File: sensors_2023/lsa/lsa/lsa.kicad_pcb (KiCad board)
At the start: 2 copper layers, 61.7 x 22.7 mm, 39 parts, among them J1 Conn_01x07_Male, U1 TCRT5000, U2 TCRT5000, U3 TCRT5000, U4 TCRT5000, U5 TCRT5000

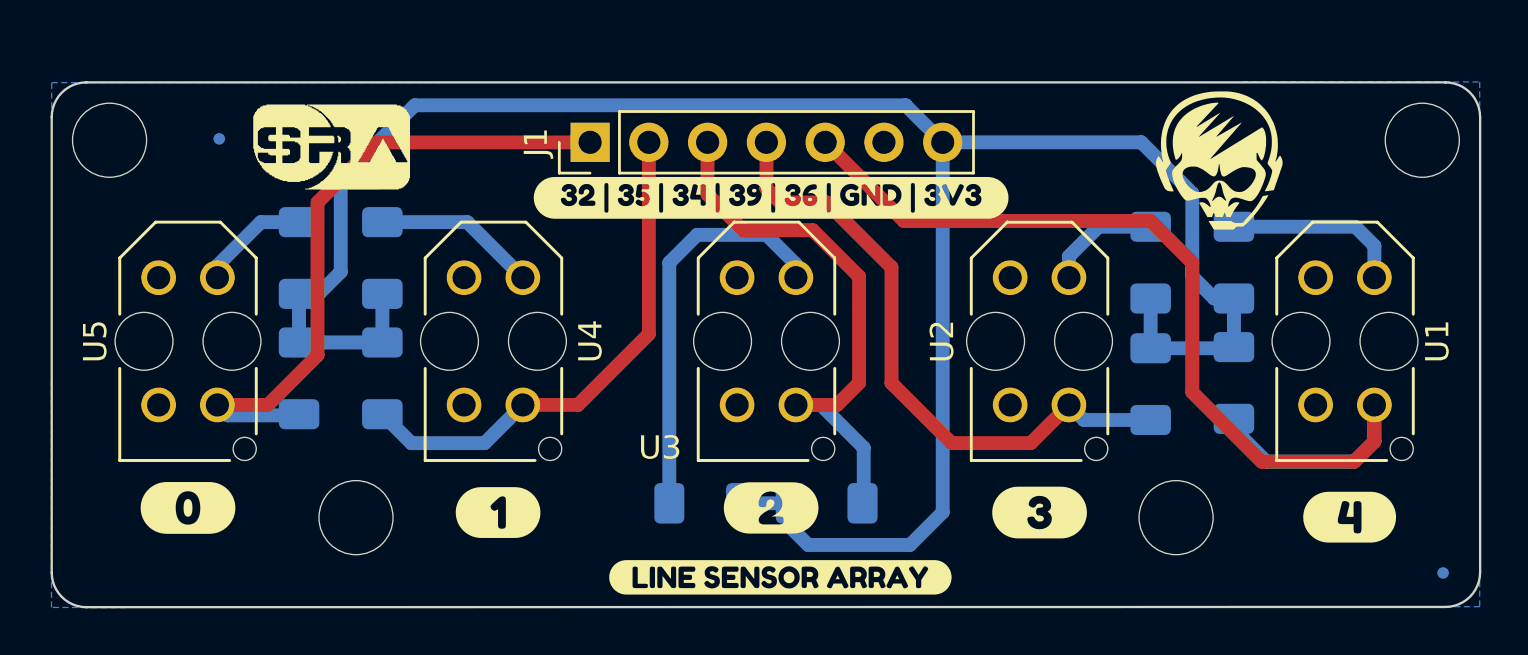
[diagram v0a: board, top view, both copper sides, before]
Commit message: Updated working content for sra_dev_board_2023
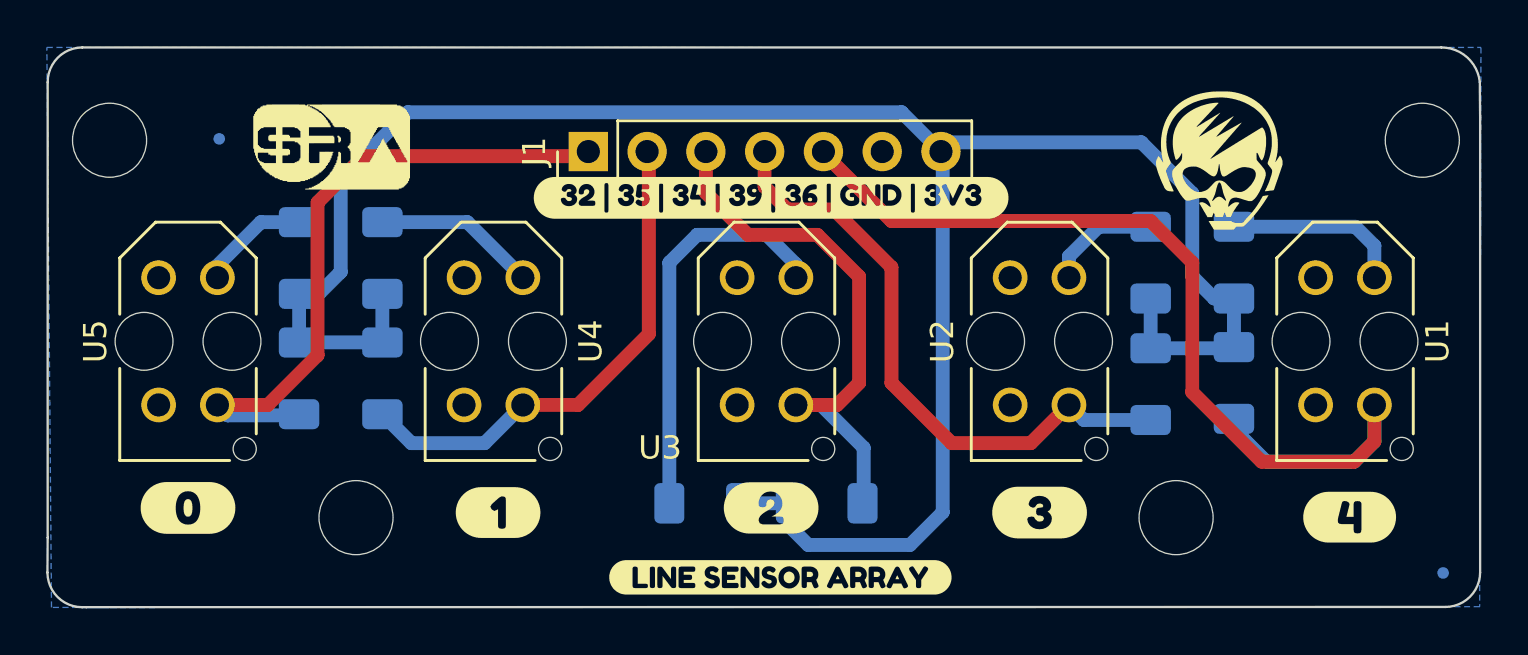
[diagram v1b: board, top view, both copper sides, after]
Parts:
- moved J1 0.41 mm to (108.5, 72.4)
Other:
- board size 61.7 x 22.7 mm -> 61.9 x 24.2 mm
